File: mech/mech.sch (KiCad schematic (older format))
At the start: 50 parts, among them P1 Pump_Motor_DC, P2 Pump_Motor_DC, T1 DS18B20, T2 DS18B20, U1 DHT22, U2 PCA9685PW, U3 ADC128D818, U4 ADC128D818

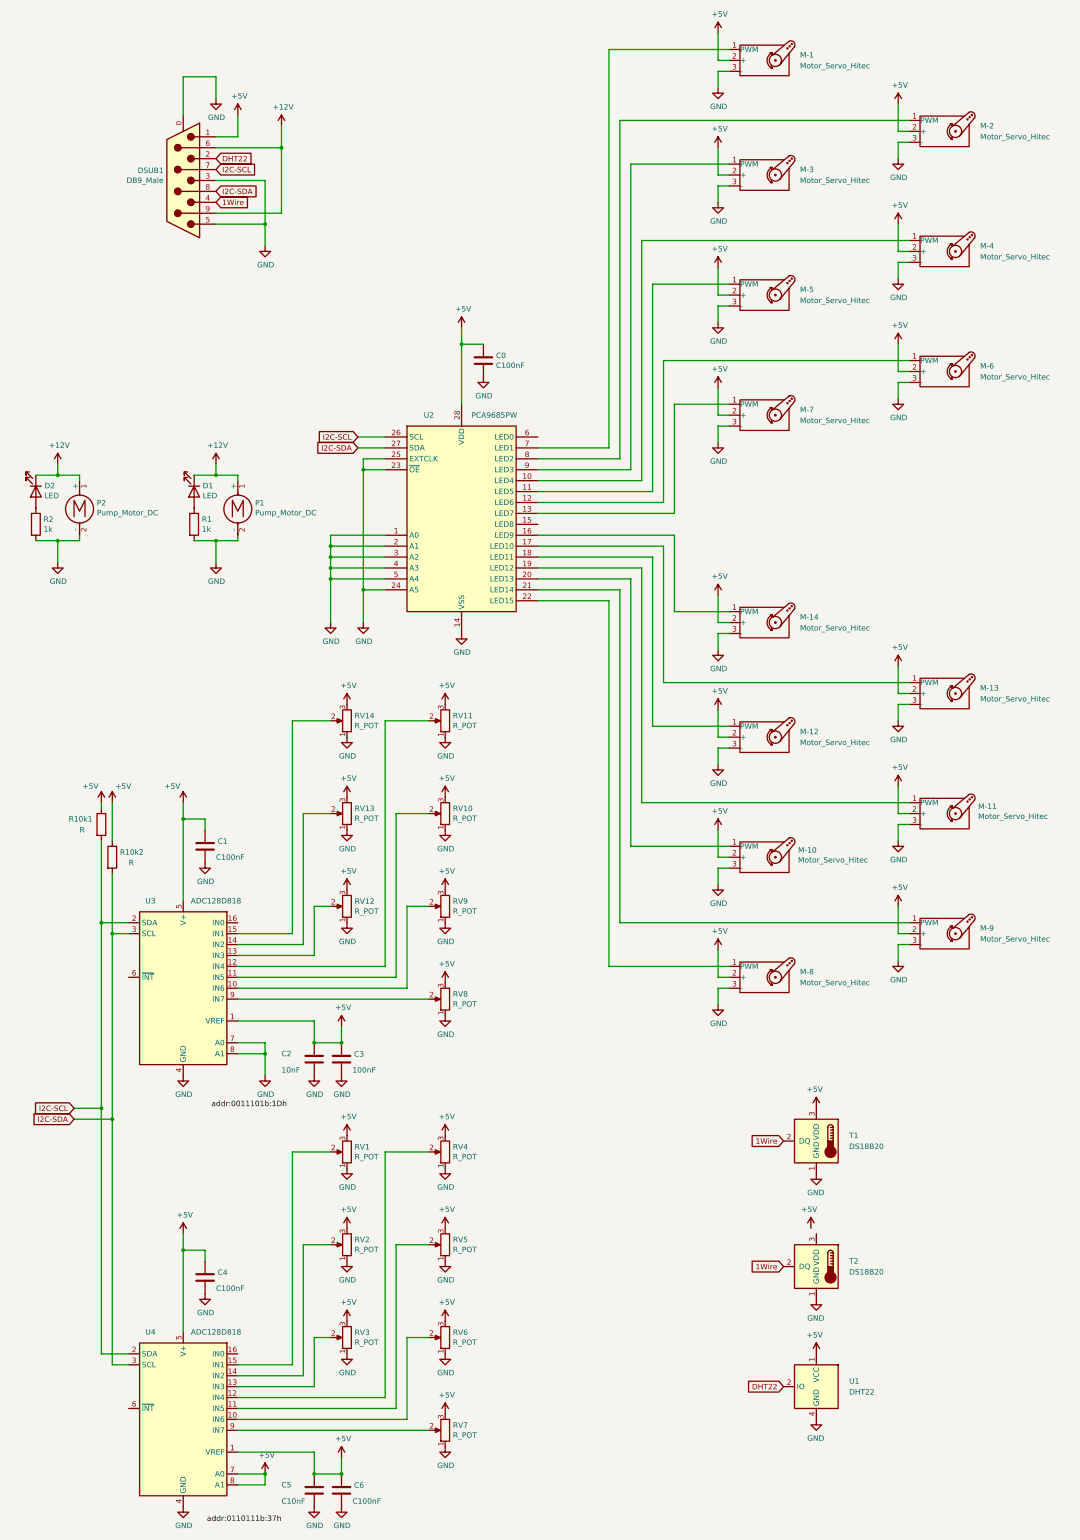
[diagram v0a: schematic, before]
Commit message: WIP sensor PCB - delete files
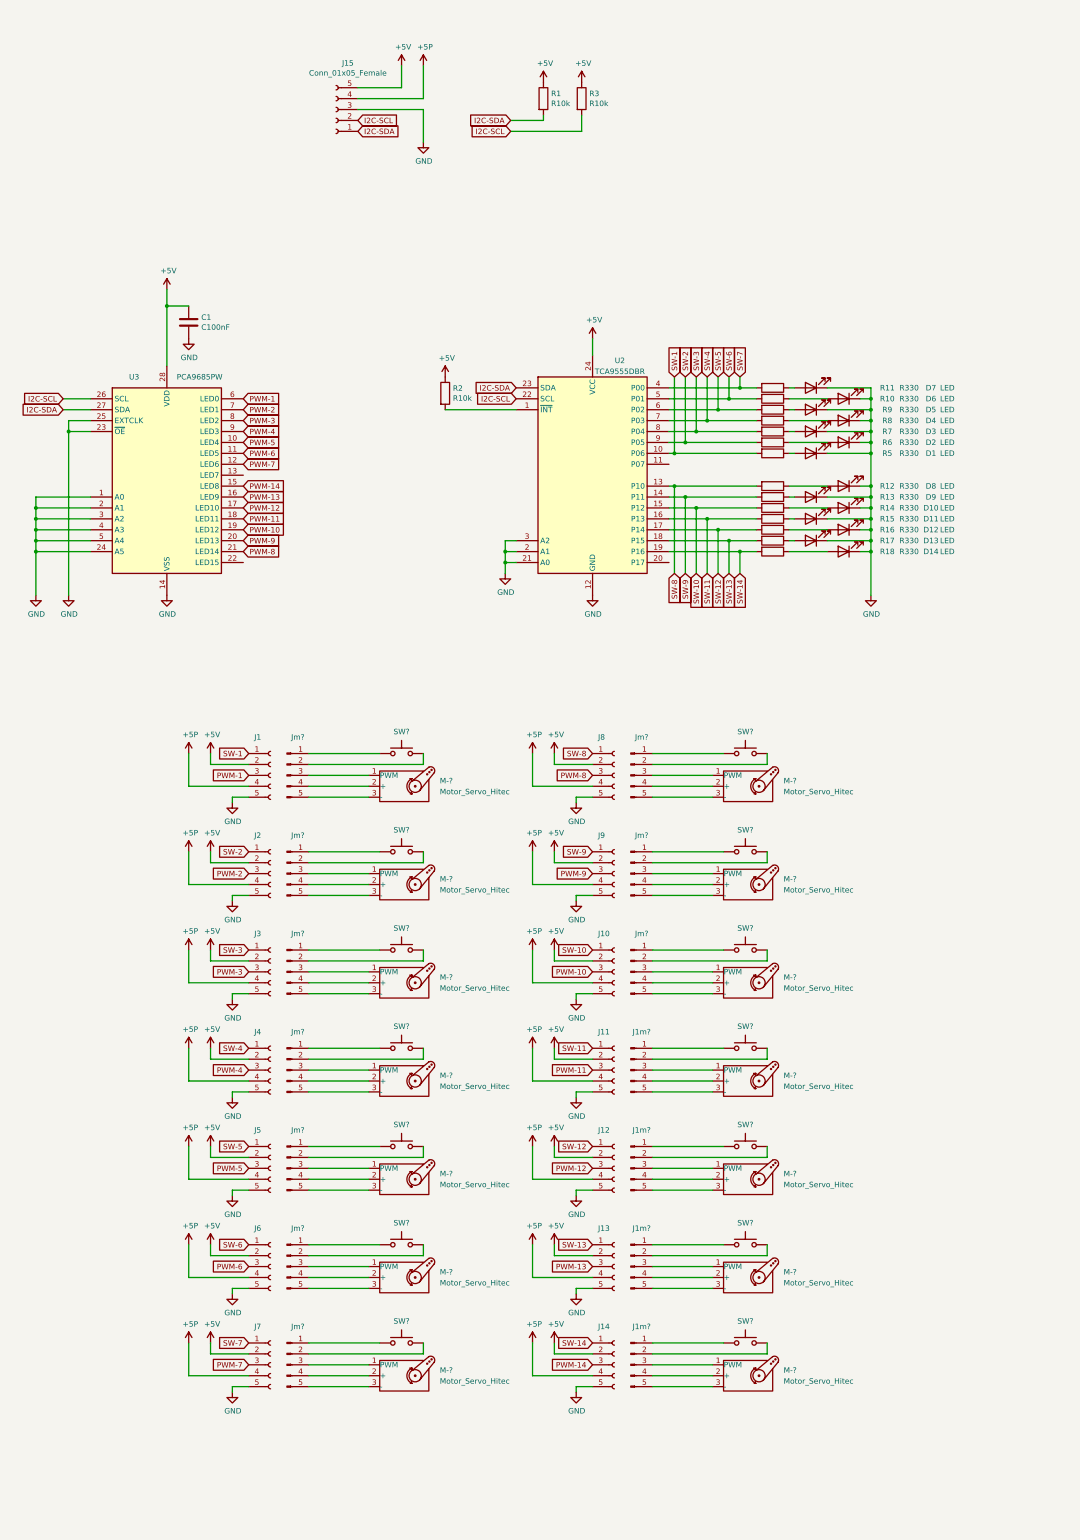
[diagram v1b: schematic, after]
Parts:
- removed C1, C4, C6: C100nF, Resistor_SMD:R_0603_1608Metric_Pad1.05x0.95mm_HandSolder, symbol Device:C
- removed C2: 10nF, Resistor_SMD:R_0603_1608Metric_Pad1.05x0.95mm_HandSolder, symbol Device:C
- removed C3: 100nF, Resistor_SMD:R_0603_1608Metric_Pad1.05x0.95mm_HandSolder, symbol Device:C
- removed C5: C10nF, Resistor_SMD:R_0603_1608Metric_Pad1.05x0.95mm_HandSolder, symbol Device:C
- removed DSUB1: DB9_Male, Connector_Dsub:DSUB-9_Male_Horizontal_P2.77x2.84mm_EdgePinOffset7.70mm_Housed_MountingHolesOffset9.12mm, symbol Connector:DB9_Male_MountingHoles
- removed M-1, M-10, M-11, M-12, M-13, M-14, M-2, M-3, M-4, M-5, M-6, M-7, M-8, M-9: Motor_Servo_Hitec, Connector_PinHeader_2.54mm:PinHeader_1x03_P2.54mm_Vertical, symbol Motor:Motor_Servo_Hitec
- removed P1, P2: Pump_Motor_DC, Connector_JST:JST_EH_B2B-EH-A_1x02_P2.50mm_Vertical, symbol Motor:Motor_DC
- removed R10k1, R10k2: R, Resistor_SMD:R_0603_1608Metric_Pad1.05x0.95mm_HandSolder, symbol Device:R
- removed RV1, RV10, RV11, RV12, RV13, RV14, RV2, RV3, RV4, RV5, RV6, RV7, RV8, RV9: R_POT, Connector_PinHeader_2.54mm:PinHeader_1x03_P2.54mm_Vertical, symbol Device:R_POT
- removed T1, T2: DS18B20, Package_TO_SOT_THT:TO-92_Inline_Wide, symbol Sensor_Temperature:DS18B20
- removed U1: DHT22, Sensor:Aosong_DHT11_5.5x12.0_P2.54mm, symbol Sensor:DHT11
- removed U3, U4: ADC128D818, Package_SO:TSSOP-16_4.4x5mm_P0.65mm, symbol Analog_ADC:ADC128D818
- added D10, D11, D12, D13, D14, D3, D4, D5, D6, D7, D8, D9: LED, LED_SMD:LED_0805_2012Metric_Pad1.15x1.40mm_HandSolder, symbol Device:LED
- added J1, J10, J11, J12, J13, J14, J2, J3, J4, J5, J6, J7, J8, J9: Conn_01x05_Female, Stardust:691382000005, symbol Connector:Conn_01x05_Female
- added J15: Conn_01x05_Female, Stardust:691382030005, symbol Connector:Conn_01x05_Female
- added J1m? (x4), Jm? (x10): Conn_01x05_Male, symbol Connector:Conn_01x05_Male
- added M-? (x14): Motor_Servo_Hitec, Connector_PinHeader_2.54mm:PinHeader_1x03_P2.54mm_Vertical, symbol Motor:Motor_Servo_Hitec
- added R10, R11, R12, R13, R14, R15, R16, R17, R18, R5, R6, R7, R8, R9: R330, Resistor_SMD:R_0603_1608Metric, symbol Device:R
- added R3: R10k, Resistor_SMD:R_0603_1608Metric_Pad0.98x0.95mm_HandSolder, symbol Device:R
- added SW? (x14): SW_Push, symbol Switch:SW_Push
- added U2: TCA9555DBR, Package_SO:SSOP-24_5.3x8.2mm_P0.65mm, symbol Interface_Expansion:TCA9555DBR
- C1: renamed from C0; footprint Resistor_SMD:R_0603_1608Metric_Pad1.05x0.95mm_HandSolder -> Resistor_SMD:R_0603_1608Metric_Pad0.98x0.95mm_HandSolder
- D1, D2: footprint Resistor_SMD:R_0603_1608Metric_Pad1.05x0.95mm_HandSolder -> LED_SMD:LED_0805_2012Metric_Pad1.15x1.40mm_HandSolder
- R1, R2: value 1k -> R10k; footprint Resistor_SMD:R_0603_1608Metric_Pad1.05x0.95mm_HandSolder -> Resistor_SMD:R_0603_1608Metric_Pad0.98x0.95mm_HandSolder
- renumbered U2 to U3
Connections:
- net +12V is gone; now on net GND: D1.1 (K), D2.1 (K)
- net +5V: now also R1.1, R2.1, J1.2 (Pin_2), J10.2 (Pin_2), J11.2 (Pin_2), J12.2 (Pin_2), J13.2 (Pin_2), J14.2 (Pin_2), J15.5 (Pin_5), J2.2 (Pin_2), J3.2 (Pin_2), J4.2 (Pin_2), J5.2 (Pin_2), J6.2 (Pin_2), J7.2 (Pin_2), J8.2 (Pin_2), J9.2 (Pin_2), R3.1, U2.24 (VCC)
- net GND: now also D10.1 (K), D11.1 (K), D12.1 (K), D13.1 (K), D14.1 (K), D3.1 (K), D4.1 (K), D5.1 (K), D6.1 (K), D7.1 (K), D8.1 (K), D9.1 (K), J1.5 (Pin_5), J10.5 (Pin_5), J11.5 (Pin_5), J12.5 (Pin_5), J13.5 (Pin_5), J14.5 (Pin_5), J15.3 (Pin_3), J2.5 (Pin_5), J3.5 (Pin_5), J4.5 (Pin_5), J5.5 (Pin_5), J6.5 (Pin_5), J7.5 (Pin_5), J8.5 (Pin_5), J9.5 (Pin_5), U2.12 (GND), U2.2 (A1), U2.21 (A0), U2.3 (A2); no longer R1.2, R2.2
- net I2C-SCL: now also J15.2 (Pin_2), R3.2, U2.22 (SCL)
- net I2C-SDA: now also R1.2, J15.1 (Pin_1), U2.23 (SDA)
- net PWM-2: now reaches U3.7 (LED1)
- net PWM-2: now also J2.3 (Pin_3)
- net PWM-4: now reaches U3.9 (LED3)
- net PWM-4: now also J4.3 (Pin_3)
- net PWM-3: now reaches U3.8 (LED2)
- net PWM-3: now also J3.3 (Pin_3)
- net PWM-6: now reaches U3.11 (LED5)
- net PWM-6: now also J6.3 (Pin_3)
- net PWM-5: now reaches U3.10 (LED4)
- net PWM-5: now also J5.3 (Pin_3)
- net PWM-7: now reaches U3.12 (LED6)
- net PWM-7: now also J7.3 (Pin_3)
- net PWM-13: now reaches U3.16 (LED9)
- net PWM-13: now also J13.3 (Pin_3)
- net PWM-12: now reaches U3.17 (LED10)
- net PWM-12: now also J12.3 (Pin_3)
- net PWM-11: now reaches U3.18 (LED11)
- net PWM-11: now also J11.3 (Pin_3)
- net PWM-10: now reaches U3.19 (LED12)
- net PWM-10: now also J10.3 (Pin_3)
- net PWM-9: now reaches U3.20 (LED13)
- net PWM-9: now also J9.3 (Pin_3)
- net at D2.2 (A): now also R6.1; no longer R2.1
- net PWM-8: now reaches U3.21 (LED14)
- net PWM-8: now also J8.3 (Pin_3)
- net at D1.2 (A): now also R5.1; no longer R1.1
- net PWM-14: now reaches U3.15 (LED8)
- net PWM-14: now also J14.3 (Pin_3)
- net PWM-1: now reaches U3.6 (LED0)
- net PWM-1: now also J1.3 (Pin_3)
- new net: D9.2 (A), R13.1
- new net: D10.2 (A), R14.1
- new net: D11.2 (A), R15.1
- new net: D12.2 (A), R16.1
- new net: D13.2 (A), R17.1
- new net: D14.2 (A), R18.1
- new net: R2.2, U2.1 (~INT)
- new net: D3.2 (A), R7.1
- new net: D4.2 (A), R8.1
- new net: D5.2 (A), R9.1
- new net: D6.2 (A), R10.1
- new net: D7.2 (A), R11.1
- new net: D8.2 (A), R12.1
- new net: Jm?.1 (Pin_1), SW?.1 (x10)
- new net: Jm?.2 (Pin_2), SW?.2 (x10)
- new net: Jm?.3 (Pin_3), M-?.1 (PWM) (x10)
- new net: Jm?.4 (Pin_4), M-?.2 (+) (x10)
- new net: Jm?.5 (Pin_5), M-?.3 (-) (x10)
- new net: J1m?.1 (Pin_1), SW?.1 (x4)
- new net: J1m?.2 (Pin_2), SW?.2 (x4)
- new net: J1m?.3 (Pin_3), M-?.1 (PWM) (x4)
- new net: J1m?.4 (Pin_4), M-?.2 (+) (x4)
- new net: J1m?.5 (Pin_5), M-?.3 (-) (x4)
- new net +5P: J1.4 (Pin_4), J10.4 (Pin_4), J11.4 (Pin_4), J12.4 (Pin_4), J13.4 (Pin_4), J14.4 (Pin_4), J15.4 (Pin_4), J2.4 (Pin_4), J3.4 (Pin_4), J4.4 (Pin_4), J5.4 (Pin_4), J6.4 (Pin_4), J7.4 (Pin_4), J8.4 (Pin_4), J9.4 (Pin_4)
- new net SW-1: J1.1 (Pin_1), R5.2, U2.10 (P06)
- new net SW-10: J10.1 (Pin_1), R14.2, U2.15 (P12)
- new net SW-11: J11.1 (Pin_1), R15.2, U2.16 (P13)
- new net SW-12: J12.1 (Pin_1), R16.2, U2.17 (P14)
- new net SW-13: J13.1 (Pin_1), R17.2, U2.18 (P15)
- new net SW-14: J14.1 (Pin_1), R18.2, U2.19 (P16)
- new net SW-2: J2.1 (Pin_1), R6.2, U2.9 (P05)
- new net SW-3: J3.1 (Pin_1), R7.2, U2.8 (P04)
- new net SW-4: J4.1 (Pin_1), R8.2, U2.7 (P03)
- new net SW-5: J5.1 (Pin_1), R9.2, U2.6 (P02)
- new net SW-6: J6.1 (Pin_1), R10.2, U2.5 (P01)
- new net SW-7: J7.1 (Pin_1), R11.2, U2.4 (P00)
- new net SW-8: J8.1 (Pin_1), R12.2, U2.13 (P10)
- new net SW-9: J9.1 (Pin_1), R13.2, U2.14 (P11)
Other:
- moved on the sheet: C1, U3
